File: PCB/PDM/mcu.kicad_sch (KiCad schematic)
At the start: 1 part, among them U1 STM32F405RGTx

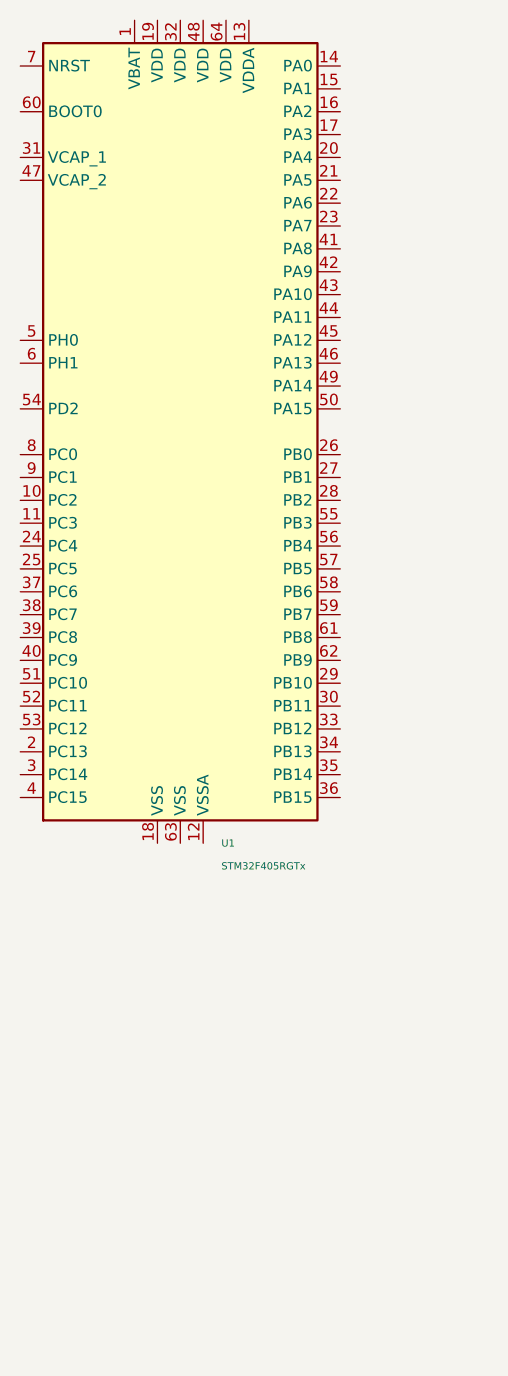
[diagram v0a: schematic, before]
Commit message: Fuck christmas & low side section
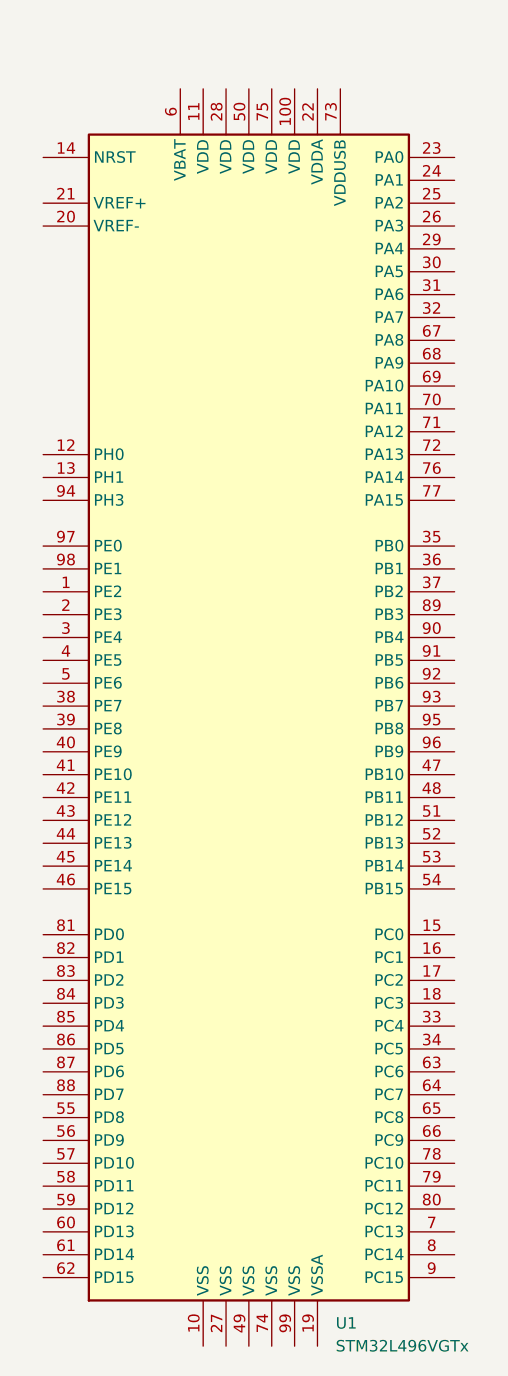
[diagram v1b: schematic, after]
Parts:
- removed U1: STM32F405RGTx, Package_QFP:LQFP-64_10x10mm_P0.5mm, symbol MCU_ST_STM32F4:STM32F405RGTx
- added U1: STM32L496VGTx, Package_QFP:LQFP-100_14x14mm_P0.5mm, symbol MCU_ST_STM32L4:STM32L496VGTx
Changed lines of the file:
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@@
 (kicad_sch (version 20211123) (generator eeschema)
   (paper "A4")
-  (symbol (lib_id "MCU_ST_STM32F4:STM32F405RGTx") (at 67.945 74.93 0) (unit 1)
+  (symbol (lib_id "MCU_ST_STM32L4:STM32L496VGTx") (at 75.565 105.41 0) (unit 1)
     (in_bom yes) (on_board yes) (fields_autoplaced)
-    (property "Reference" "U1" (id 0) (at 72.5044 120.65 0)
-      (effects (font (size 0.8 0.8)) (justify left))
+    (property "Reference" "U1" (id 0) (at 85.2044 173.99 0)
+      (effects (font (size 1.27 1.27)) (justify left))
     )
-    (property "Value" "STM32F405RGTx" (id 1) (at 72.5044 123.19 0)
-      (effects (font (size 0.8 0.8)) (justify left))
+    (property "Value" "STM32L496VGTx" (id 1) (at 85.2044 176.53 0)
+      (effects (font (size 1.27 1.27)) (justify left))
     )
-    (property "Footprint" "Package_QFP:LQFP-64_10x10mm_P0.5mm" (id 2) (at 52.705 118.11 0)
+    (property "Footprint" "Package_QFP:LQFP-100_14x14mm_P0.5mm" (id 2) (at 57.785 171.45 0)
       (effects (font (size 1.27 1.27)) (justify right) hide)
     )
-    (property "Datasheet" "http://www.st.com/st-web-ui/static/active/en/resource/technical/document/datasheet/DM00037051.pdf" (id 3) (at 67.945 74.93 0)
+    (property "Datasheet" "http://www.st.com/st-web-ui/static/active/en/resource/technical/document/datasheet/DM00284211.pdf" (id 3) (at 75.565 105.41 0)
       (effects (font (size 1.27 1.27)) hide)
     )
     (pin "1")
     (pin "10")
+    (pin "100")
     (pin "11")
     (pin "12")
@@
     (pin "63")
     (pin "64")
+    (pin "65")
+    (pin "66")
+    (pin "67")
+    (pin "68")
+    (pin "69")
     (pin "7")
+    (pin "70")
+    (pin "71")
+    (pin "72")
+    (pin "73")
+    (pin "74")
+    (pin "75")
+    (pin "76")
+    (pin "77")
+    (pin "78")
+    (pin "79")
     (pin "8")
+    (pin "80")
+    (pin "81")
+    (pin "82")
+    (pin "83")
+    (pin "84")
+    (pin "85")
+    (pin "86")
+    (pin "87")
+    (pin "88")
+    (pin "89")
     (pin "9")
+    (pin "90")
+    (pin "91")
+    (pin "92")
+    (pin "93")
+    (pin "94")
+    (pin "95")
+    (pin "96")
+    (pin "97")
+    (pin "98")
+    (pin "99")
   )
 )
